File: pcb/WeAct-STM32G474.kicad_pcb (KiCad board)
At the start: 2 copper layers, 50 x 40 mm, 36 parts, among them J3 P1, J4 P2, U1 AMS1117-3.3, U2 SRV05-4, U3 STM32G474CBTx, Y1 X_24MHZ

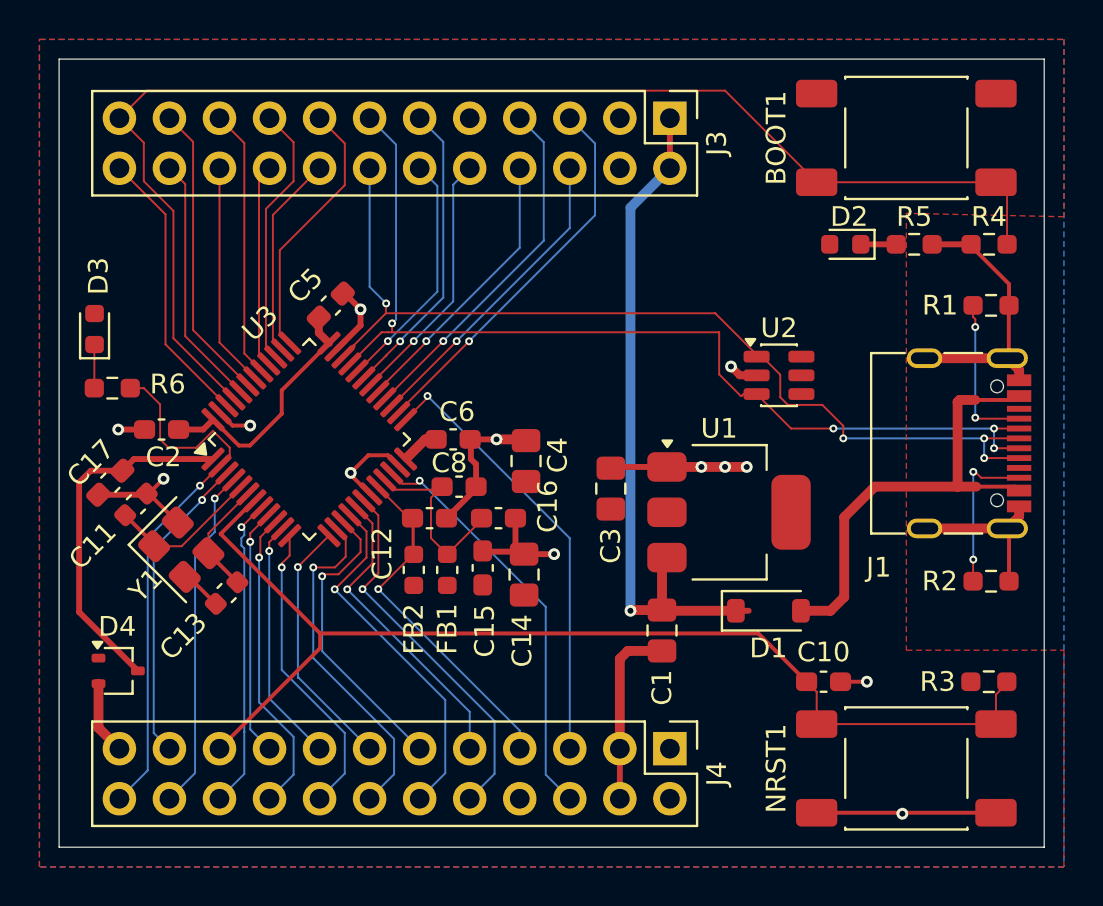
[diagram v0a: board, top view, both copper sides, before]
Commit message: pcb design phase 1
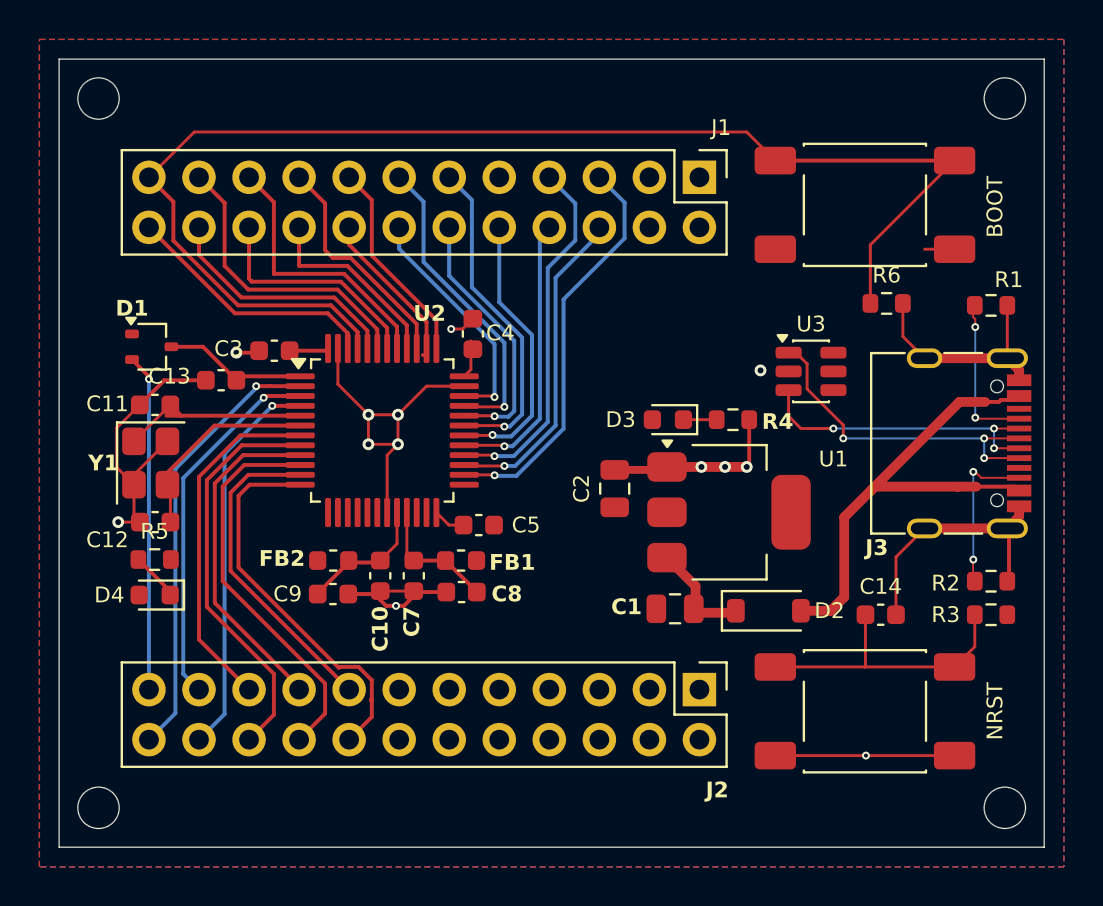
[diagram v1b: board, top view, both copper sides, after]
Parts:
- removed the C14 at (142.6, 104.2)
- removed C15, C17, C6: C_100NF_0603, Capacitor_SMD:C_0603_1608Metric_Pad1.08x0.95mm_HandSolder
- removed C16: C_1UF_0603, Capacitor_SMD:C_0603_1608Metric_Pad1.08x0.95mm_HandSolder
- added C10: C_100NF_0603, Capacitor_SMD:C_0603_1608Metric, F.Cu at (135.3, 104.2)
- added C7: C_100NF_0603, Capacitor_SMD:C_0603_1608Metric, F.Cu at (137.0, 104.2)
- added C9: C_1UF_0603, Capacitor_SMD:C_0603_1608Metric, F.Cu at (132.9, 105.2)
- added REF**: MountingHole_2.1mm, MountingHole:MountingHole_2.1mm, F.Cu at (121.0, 116.0)
- added REF**: MountingHole_2.1mm, MountingHole:MountingHole_2.1mm, F.Cu at (167.0, 116.0)
- added REF**: MountingHole_2.1mm, MountingHole:MountingHole_2.1mm, F.Cu at (121.0, 80.0)
- added REF**: MountingHole_2.1mm, MountingHole:MountingHole_2.1mm, F.Cu at (167.0, 80.0)
- C1: footprint Capacitor_SMD:C_0805_2012Metric_Pad1.18x1.45mm_HandSolder -> Capacitor_SMD:C_0805_2012Metric
- C12: value C_100NF_0603 -> C_20PF_0603; footprint Capacitor_SMD:C_0603_1608Metric_Pad1.08x0.95mm_HandSolder -> Capacitor_SMD:C_0603_1608Metric
- C13: value C_20PF_0603 -> C_100NF_0603
- C14: renamed from C10; footprint Capacitor_SMD:C_0603_1608Metric_Pad1.08x0.95mm_HandSolder -> Capacitor_SMD:C_0603_1608Metric
- C2: value C_100NF_0603 -> C_10UF_0805; footprint Capacitor_SMD:C_0603_1608Metric_Pad1.08x0.95mm_HandSolder -> Capacitor_SMD:C_0805_2012Metric
- C3: value C_10UF_0805 -> C_1UF_0805; footprint Capacitor_SMD:C_0805_2012Metric_Pad1.18x1.45mm_HandSolder -> Capacitor_SMD:C_0603_1608Metric
- C4: value C_1UF_0805 -> C_100NF_0603; footprint Capacitor_SMD:C_0805_2012Metric_Pad1.18x1.45mm_HandSolder -> Capacitor_SMD:C_0603_1608Metric
- C5: footprint Capacitor_SMD:C_0603_1608Metric_Pad1.08x0.95mm_HandSolder -> Capacitor_SMD:C_0603_1608Metric
- C8: value C_100NF_0603 -> C_1UF_0603; footprint Capacitor_SMD:C_0603_1608Metric_Pad1.08x0.95mm_HandSolder -> Capacitor_SMD:C_0603_1608Metric
- R1, R2, R3: footprint Resistor_SMD:R_0603_1608Metric_Pad0.98x0.95mm_HandSolder -> Resistor_SMD:R_0603_1608Metric
- R4: renamed from R5; footprint Resistor_SMD:R_0603_1608Metric_Pad0.98x0.95mm_HandSolder -> Resistor_SMD:R_0603_1608Metric
- R5: renamed from R6; footprint Resistor_SMD:R_0603_1608Metric_Pad0.98x0.95mm_HandSolder -> Resistor_SMD:R_0603_1608Metric
- R6: renamed from R4; footprint Resistor_SMD:R_0603_1608Metric_Pad0.98x0.95mm_HandSolder -> Resistor_SMD:R_0603_1608Metric
- moved C2 23.2 mm to (147.2, 99.8), turned to 90 degrees
- moved C3 18.5 mm to (129.9, 92.8), turned to 180 degrees
- moved D1 16.5 mm to (123.7, 92.6)
- moved C12 13.9 mm to (123.9, 101.5), turned to 180 degrees
- moved D4 13.8 mm to (123.8, 105.2), turned to 180 degrees
- moved C5 13.4 mm to (140.3, 101.7), turned to 0 degrees
- moved R4 12.8 mm to (153.2, 96.3)
- moved D3 12.7 mm to (149.9, 96.3)
- moved C13 10.8 mm to (127.2, 94.3), turned to 180 degrees
- moved R5 8.96 mm to (123.8, 103.4)
- moved C4 6.99 mm to (140.0, 92.0)
- moved R6 6.00 mm to (161.0, 90.4), turned to 0 degrees
- moved C8 5.35 mm to (139.4, 105.0), turned to 180 degrees
- moved C11 5.14 mm to (123.9, 95.5), turned to 180 degrees
- moved Y1 4.67 mm to (123.7, 98.5), turned to -90 degrees
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- renumbered BOOT1 to BOOT, D4 to D1, D1 to D2, D2 to D3, D3 to D4, J3 to J1, J4 to J2, J1 to J3, NRST1 to NRST, U3 to U2, U2 to U3
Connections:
- C12 pad 1: VREF -> Net-(U2-PF1)
- C13 pad 1: Net-(U3-PF1) -> VBAT
- J1 pad 1: +5V -> +3V3
- J1 pad 2: +5V -> +3V3
- J2 pad 1: +3V3 -> +5V
- J2 pad 2: +3V3 -> +5V
- U2 pad 6: Net-(U3-PF1) -> Net-(U2-PF1)
- Y1 pad 3: Net-(U3-PF1) -> Net-(U2-PF1)
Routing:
- net +5V: track 34.7 -> 5.49 mm, vias 1 -> 0
- net NRST: track 57.1 -> 32.7 mm
- net PB11: track 22.6 -> 0.00 mm, vias 1 -> 0
- net PB10: track 21.0 -> 0.00 mm, vias 1 -> 0
- net PA11: track 51.8 -> 31.5 mm
- net PA12: track 49.5 -> 29.6 mm
- net PB2: track 19.1 -> 0.00 mm, vias 1 -> 0
- net PB0: track 18.3 -> 0.00 mm, vias 1 -> 0
- net PA6: track 17.4 -> 0.00 mm, vias 1 -> 0
- net PB1: track 15.7 -> 0.00 mm, vias 1 -> 0
- net PA7: track 15.2 -> 0.00 mm, vias 1 -> 0
- net VB: track 3.74 -> 17.1 mm, vias 0 -> 1
- net PA5: track 13.1 -> 0.00 mm, vias 1 -> 0
- net VREF: track 19.7 -> 6.80 mm, vias 1 -> 0
- net VBAT: track 18.5 -> 7.33 mm
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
